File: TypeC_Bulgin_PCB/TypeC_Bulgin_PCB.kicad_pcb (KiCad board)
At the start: 2 copper layers, 16.1 x 16.1 mm, 12 parts, among them J1 Conn_01x01_Female, J10 Conn_01x01_Female, J11 Conn_01x01_Female, J12 Conn_01x01_Female, J2 Conn_01x01_Female, J3 USB_C_Receptacle, J4 Conn_01x02_Female, J5 Conn_01x02_Female, J6 Conn_01x02_Female, J7 Conn_01x02_Female, J8 Conn_01x01_Female, J9 Conn_01x01_Female

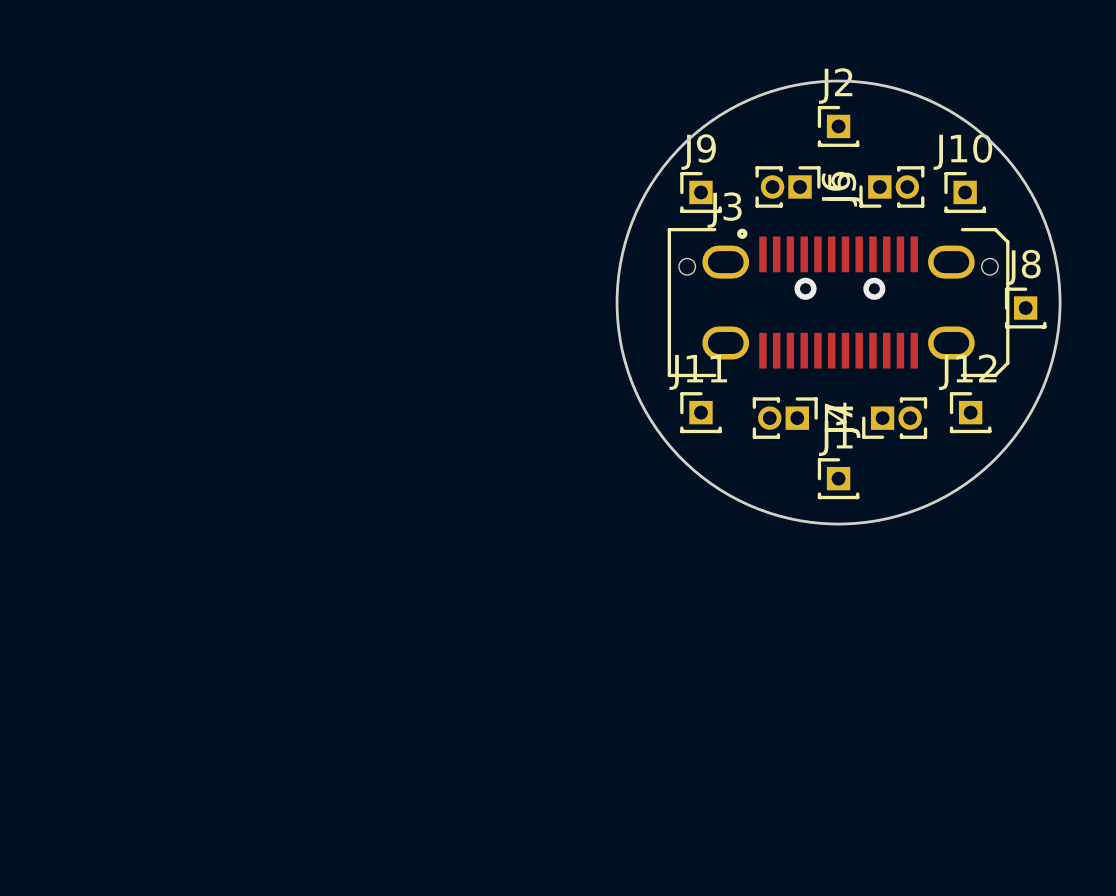
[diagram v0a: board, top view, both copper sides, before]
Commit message: v0.6 connectors prototype were added
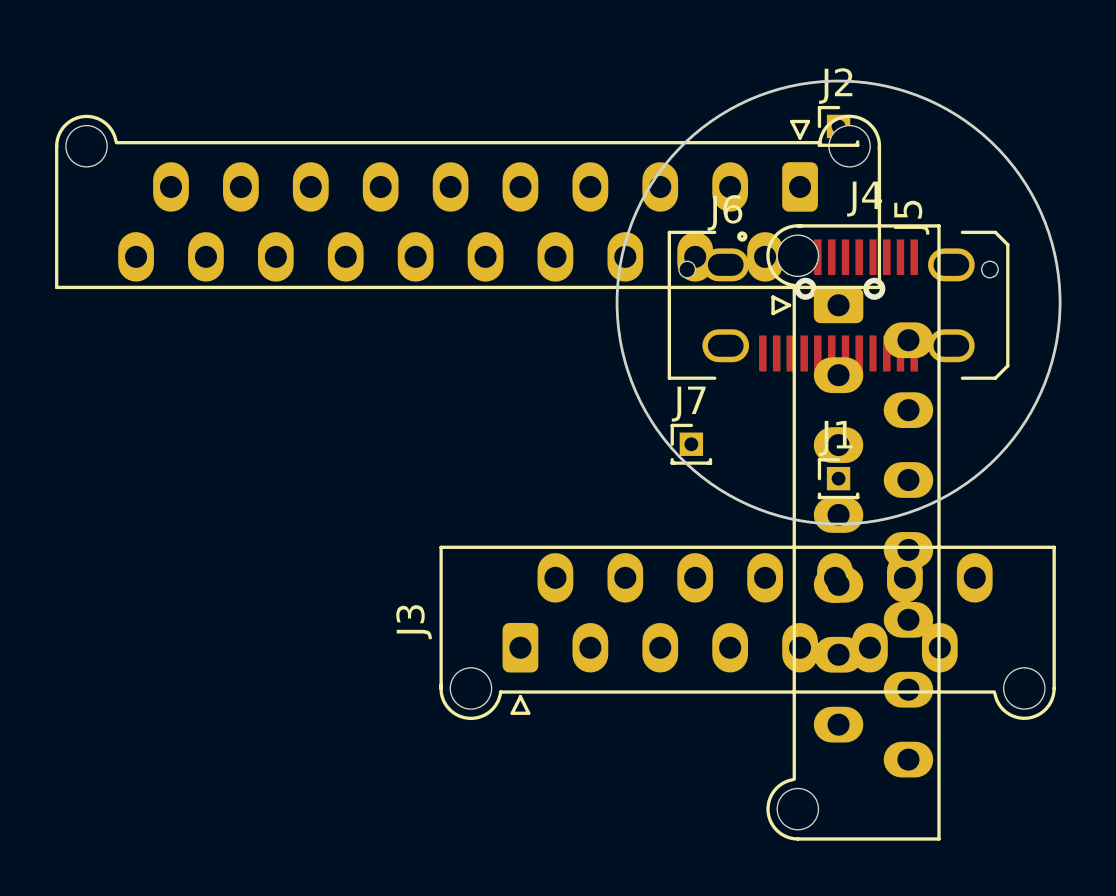
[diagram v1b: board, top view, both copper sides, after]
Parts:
- removed J10, J11, J12, J8, J9: Conn_01x01_Female, Connector_PinHeader_1.00mm:PinHeader_1x01_P1.00mm_Vertical
- J3: value USB_C_Receptacle -> Conn_01x13; footprint Connector_USB:USB_C_Receptacle_JAE_DX07S024WJ3R400 -> Connector_Molex:Molex_Picoflex_90325-0014_2x07_P1.27mm_Vertical
- J4: value Conn_01x02_Female -> Conn_01x13; footprint Connector_PinHeader_1.00mm:PinHeader_1x02_P1.00mm_Vertical -> Connector_Molex:Molex_Picoflex_90325-0014_2x07_P1.27mm_Vertical
- J5: value Conn_01x02_Female -> Conn_02x10_Odd_Even; footprint Connector_PinHeader_1.00mm:PinHeader_1x02_P1.00mm_Vertical -> Connector_Molex:Molex_Picoflex_90325-0020_2x10_P1.27mm_Vertical
- J6: value Conn_01x02_Female -> USB_C_Receptacle; footprint Connector_PinHeader_1.00mm:PinHeader_1x02_P1.00mm_Vertical -> Connector_USB:USB_C_Receptacle_JAE_DX07S024WJ3R400
- J7: value Conn_01x02_Female -> Conn_01x01_Female; footprint Connector_PinHeader_1.00mm:PinHeader_1x02_P1.00mm_Vertical -> Connector_PinHeader_1.00mm:PinHeader_1x01_P1.00mm_Vertical
- moved J3 17.1 mm to (139.6, 99.9), turned to 90 degrees
- moved J7 7.01 mm to (145.8, 92.5), turned to 0 degrees
- moved J6 4.55 mm to (151.2, 87.5), turned to 0 degrees
- moved J4 4.37 mm to (151.2, 87.5), turned to 0 degrees
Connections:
- J4 pad 1: Net-(J3-PadB10) -> VBUS
- J4 pad 2: Net-(J3-PadB11) -> VBUS
- J5 pad 1: Net-(J3-PadA3) -> GND
- J5 pad 2: Net-(J3-PadA2) -> RX1-
- J7 pad 1: Net-(J3-PadB3) -> Net-(J6-PadS1)
